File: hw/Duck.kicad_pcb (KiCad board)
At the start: 2 copper layers, 33.1 x 16.3 mm, 41 parts, among them J1 FFC P0.5, J2 Pin P2.54, J3 USB_C_Receptacle_USB2.0_14P, Q1 MMBT3904, Q2 MMBT3904, U1 ESP32-S3-PICO-1, U2 SPX3819M5-L-3-3, U3 INMP441, U4 MAX17048G+T10, U5 CH343P, U6 SPX3819M5-L-3-3

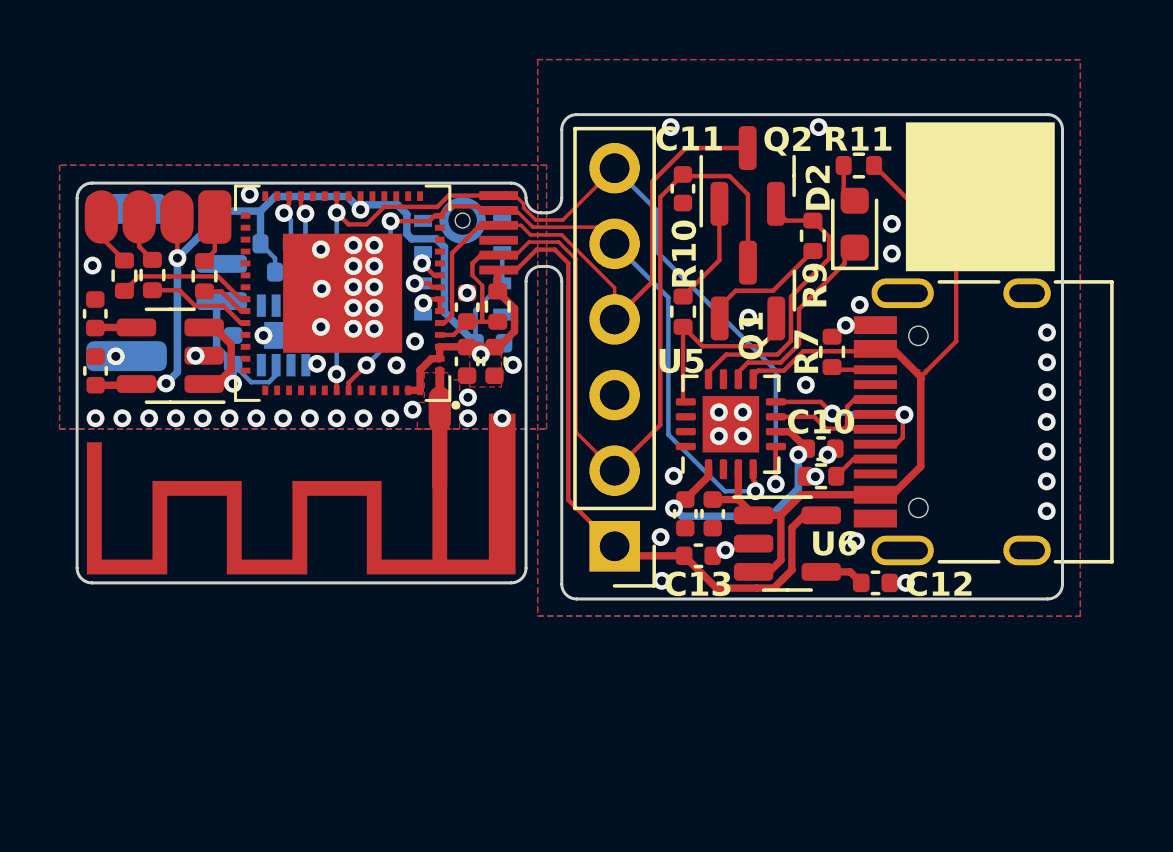
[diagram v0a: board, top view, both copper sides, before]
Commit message: hw: Final stretch; submit for fab (Rev. 2)
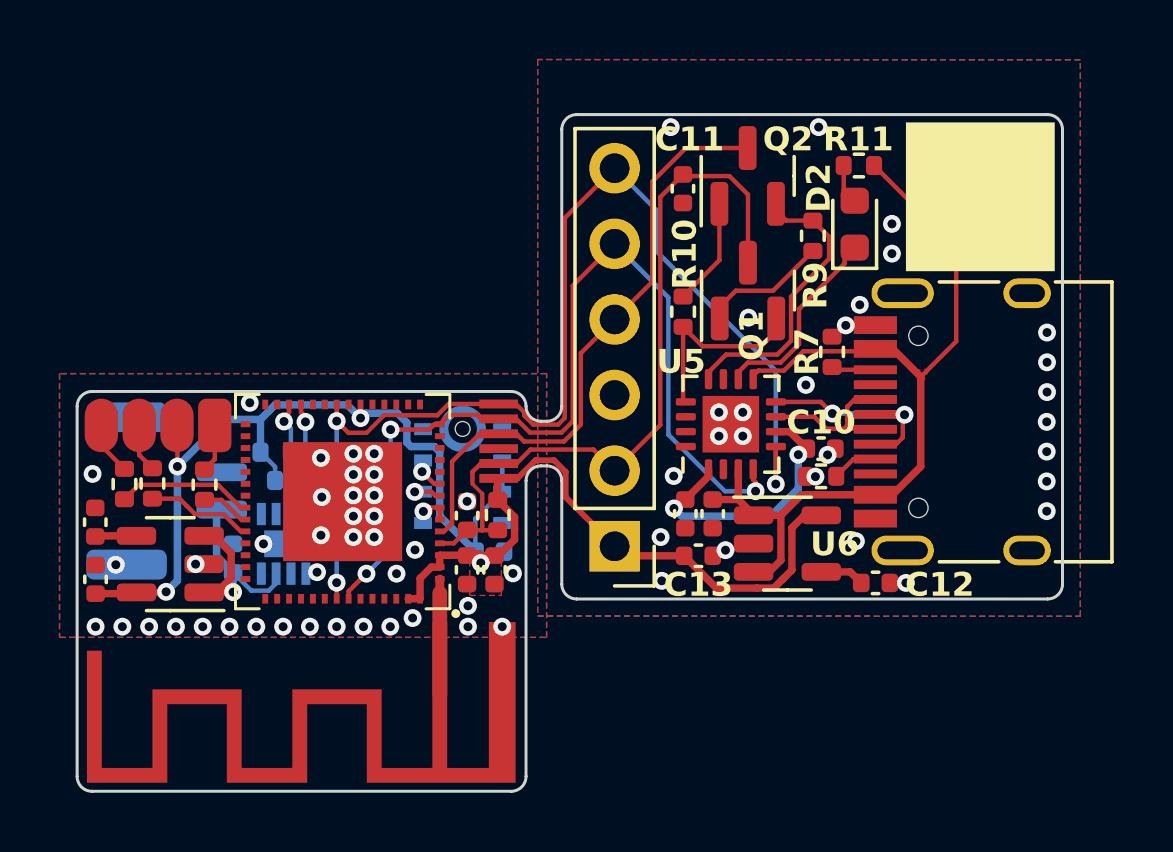
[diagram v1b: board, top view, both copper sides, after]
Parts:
- moved AE1 7.00 mm to (73.3, 56.2)
- moved BT1 7.00 mm to (62.1, 51.8)
- moved C1 7.00 mm to (73.1, 54.5)
- moved C2 7.00 mm to (72.2, 54.5)
- moved C3 7.00 mm to (72.2, 52.6)
- moved C4 7.00 mm to (59.7, 52.9)
- moved C5 7.00 mm to (59.7, 54.8)
- moved C6 7.00 mm to (72.9, 53.9)
- moved C7 7.00 mm to (64.3, 54.1)
- moved D1 7.00 mm to (61.8, 49.6)
- moved G*** 7.00 mm to (71.8, 59.3)
- moved J1 7.00 mm to (73.2, 50.1)
- moved R1 7.00 mm to (73.2, 52.6)
- moved R2 7.00 mm to (65.7, 50.5)
- moved R3 7.00 mm to (66.2, 51.5)
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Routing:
- net /U0TXD: track 31.6 -> 38.9 mm
- net +3V3: track 58.8 -> 51.6 mm
- net /ESP_EN: track 31.9 -> 25.5 mm
- net /U0RXD: track 26.3 -> 31.7 mm
- net /BOOT0: track 19.4 -> 20.7 mm
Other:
- board size 33.1 x 16.3 mm -> 33.1 x 22.7 mm
